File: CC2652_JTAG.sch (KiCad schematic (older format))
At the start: 2 parts

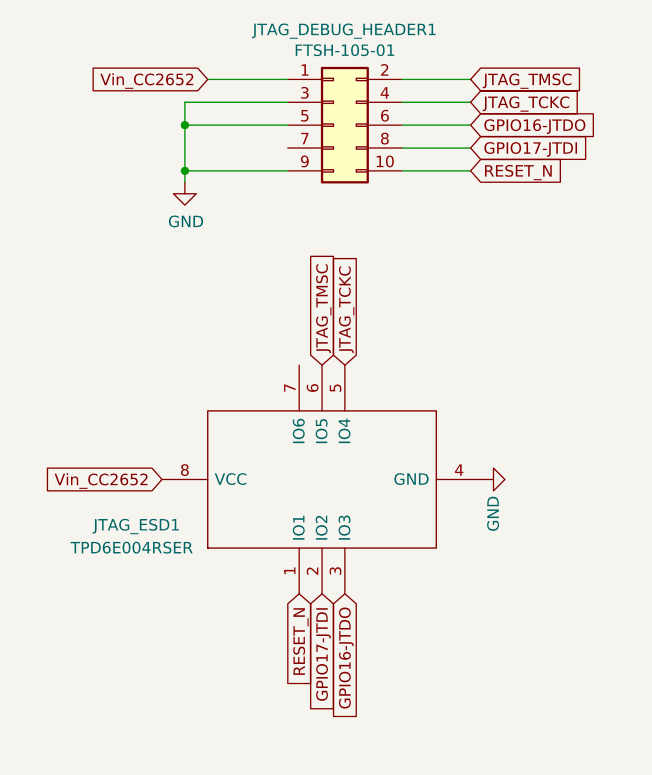
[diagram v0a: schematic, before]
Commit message: Update+UL PCB
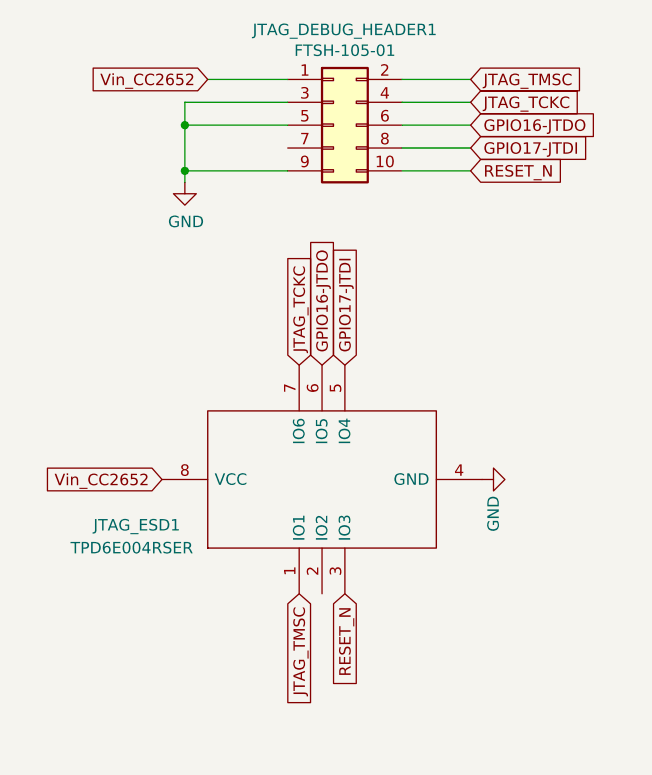
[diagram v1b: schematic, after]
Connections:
- net GPIO16-JTDO: now also JTAG_ESD1.6 (IO5); no longer JTAG_ESD1.3 (IO3)
- net GPIO17-JTDI: now also JTAG_ESD1.5 (IO4); no longer JTAG_ESD1.2 (IO2)
- net JTAG_TCKC: now also JTAG_ESD1.7 (IO6); no longer JTAG_ESD1.5 (IO4)
- net JTAG_TMSC: now also JTAG_ESD1.1 (IO1); no longer JTAG_ESD1.6 (IO5)
- net RESET_N: now also JTAG_ESD1.3 (IO3); no longer JTAG_ESD1.1 (IO1)
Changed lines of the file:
@@
 	0    -1   -1   0
 $EndComp
+Text GLabel 5800 4650 3    50   Input ~ 0
+RESET_N
+Text GLabel 5800 3650 1    50   Input ~ 0
+GPIO17-JTDI
+Text GLabel 5700 3650 1    50   Input ~ 0
+GPIO16-JTDO
+Text GLabel 5600 3650 1    50   Input ~ 0
+JTAG_TCKC
 Text GLabel 5600 4650 3    50   Input ~ 0
-RESET_N
-Text GLabel 5700 4650 3    50   Input ~ 0
-GPIO17-JTDI
-Text GLabel 5800 4650 3    50   Input ~ 0
-GPIO16-JTDO
-Text GLabel 5800 3650 1    50   Input ~ 0
-JTAG_TCKC
-Text GLabel 5700 3650 1    50   Input ~ 0
 JTAG_TMSC
 $EndSCHEMATC
